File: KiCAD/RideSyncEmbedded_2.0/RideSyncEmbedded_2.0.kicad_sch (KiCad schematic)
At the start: 76 parts, among them IC2 SIP32431DR3-T1GE3, IC3 MAX40018ATA+, IC4 SIP32432DR3-T1GE3, IC5 INA190A4QDCKRQ1, IC6 MAX40018ATA+, IC7 INA190A4QDCKRQ1, IC8 MAX40018ATA+, IC9 MAX40018ATA+, J1 Conn_01x02_Pin, J2 Conn_01x02_Pin, U1 TLV3691, U2 BQ25505RGRR, U3 BQ25505RGRR

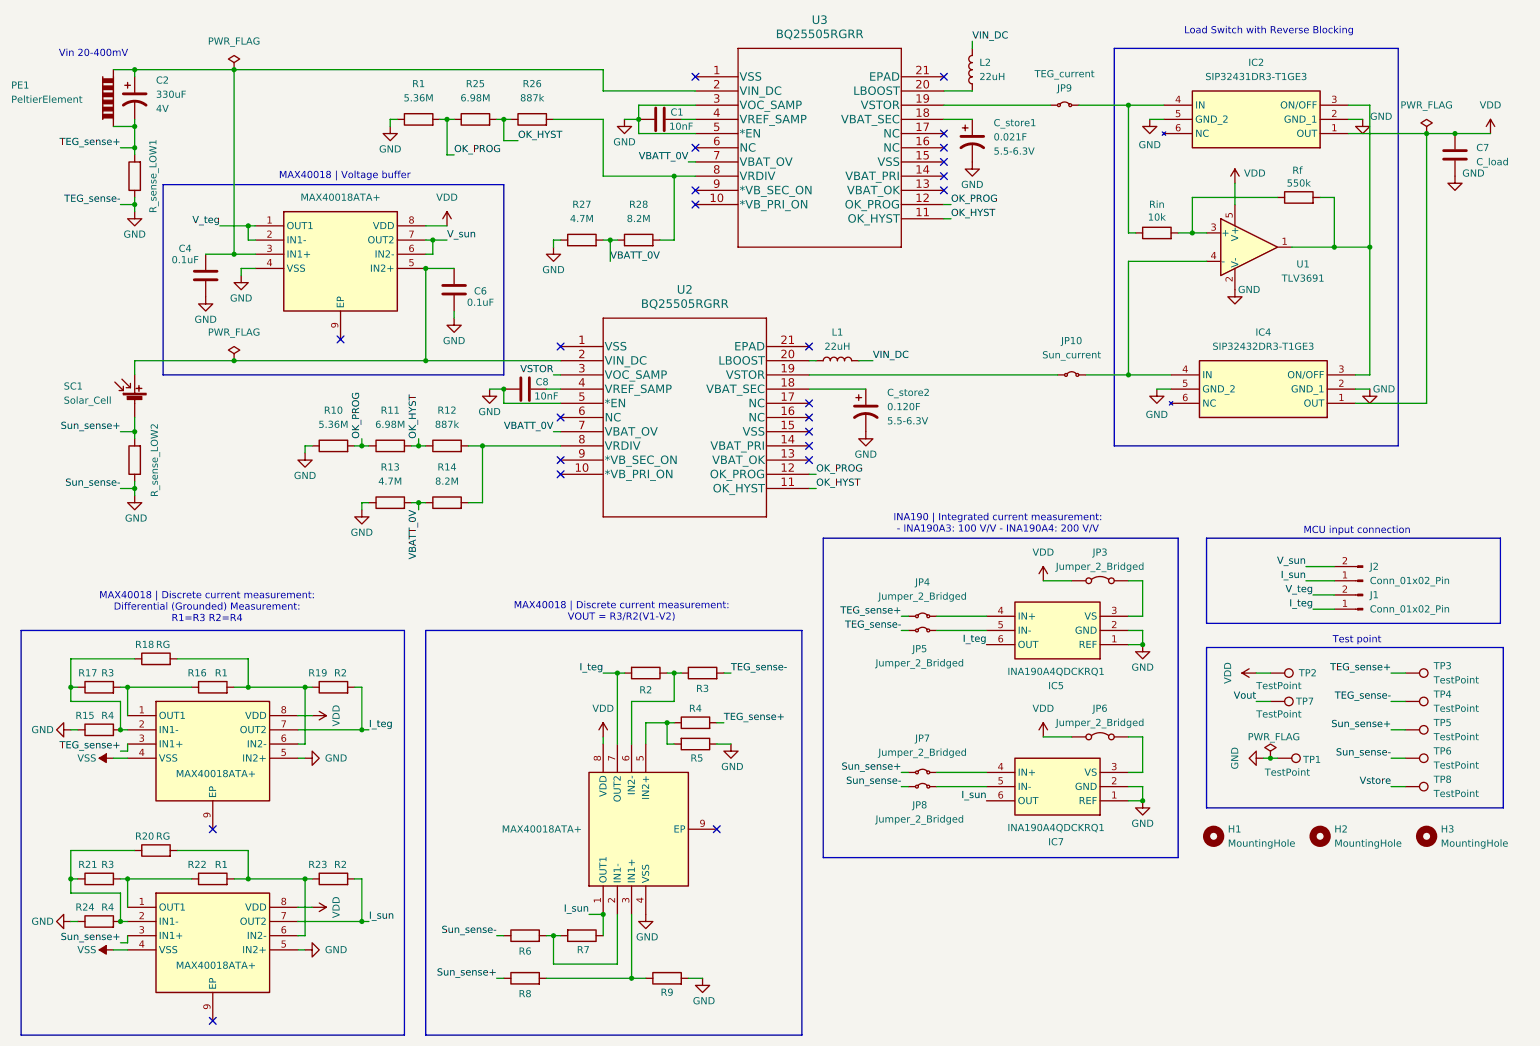
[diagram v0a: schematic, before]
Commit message: fig
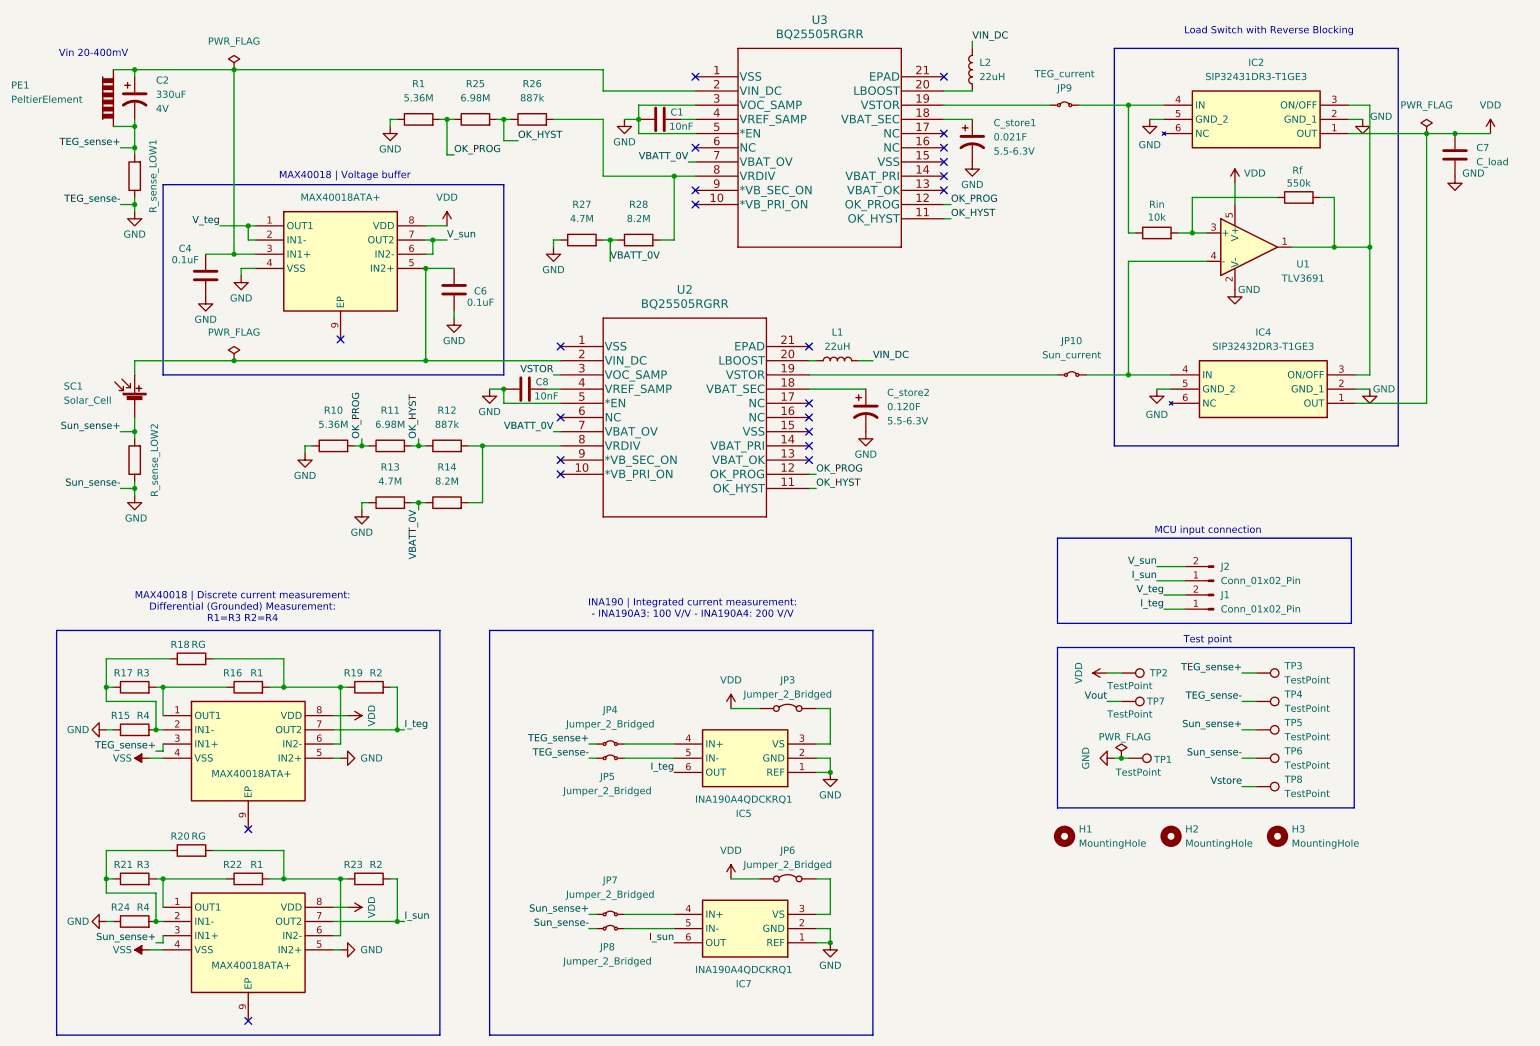
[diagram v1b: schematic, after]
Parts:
- removed IC6: MAX40018ATA+, SON65P300X300X80-9N, symbol MAX40018ATA+:MAX40018ATA+
- removed R2, R3, R4, R5, R6, R7, R8, R9: R, symbol Device:R
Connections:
- no-connect marks 24 -> 23
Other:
- note removed: "MAX40018 | Discrete current measurement: VOUT = R3/R2(V1-V2)"
- moved on the sheet: H1, H2, H3, IC5, IC7, J1, J2, JP3, JP4, JP5, JP6, JP7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
